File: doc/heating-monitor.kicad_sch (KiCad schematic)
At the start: 7 parts, among them U1 WeMos_D1_mini, U2 DS18B20, U3 DS18B20, U4 DS18B20, U5 DS18B20

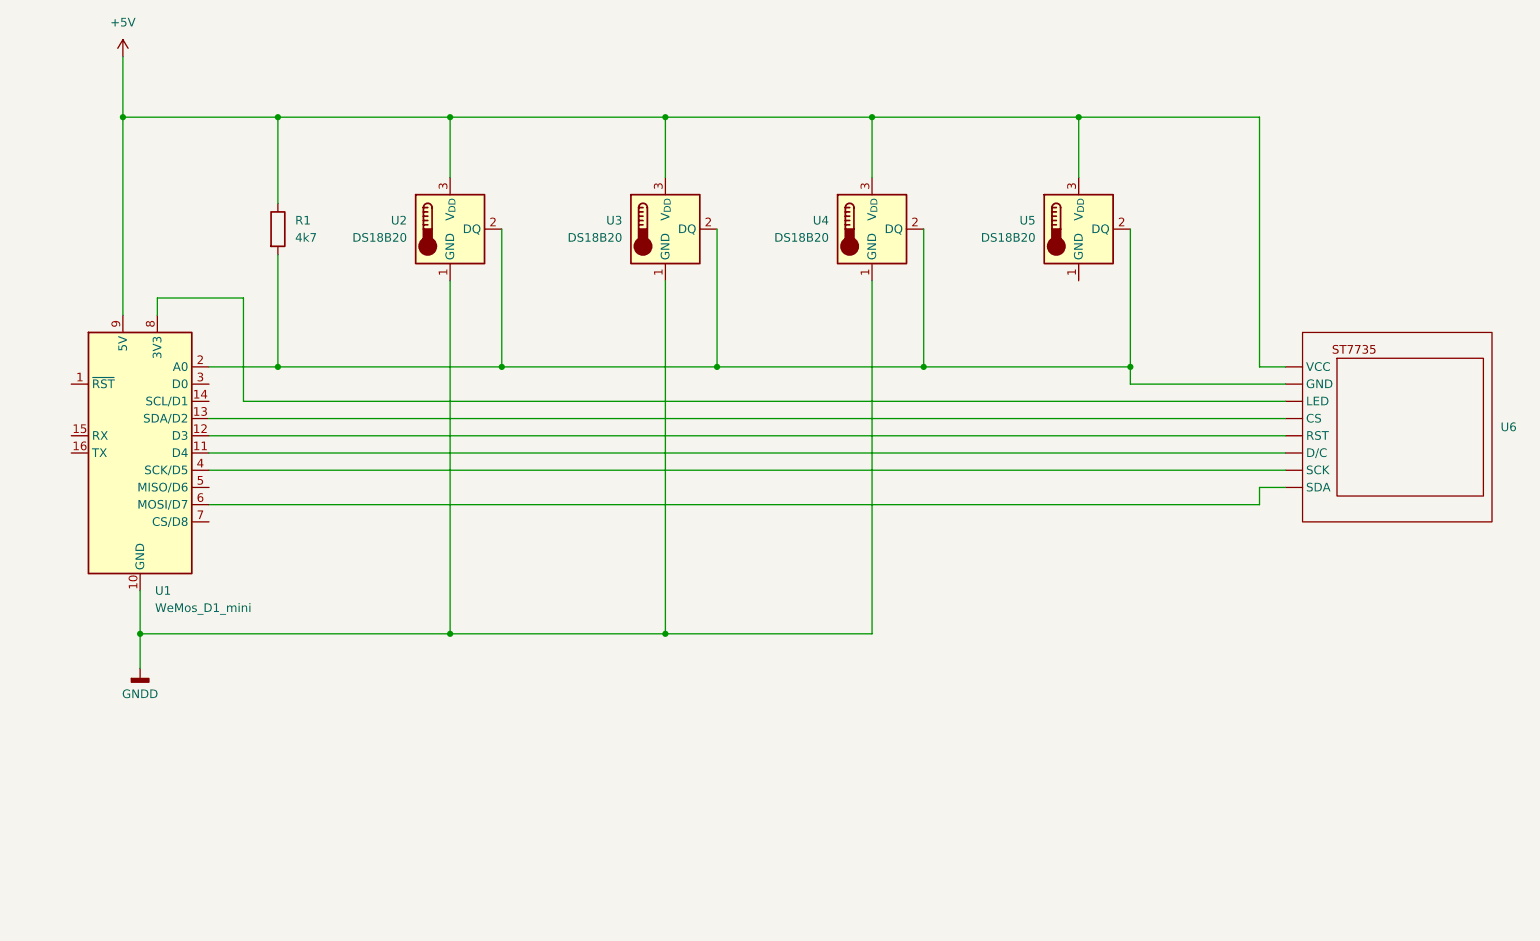
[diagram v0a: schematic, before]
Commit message: Updated schematic
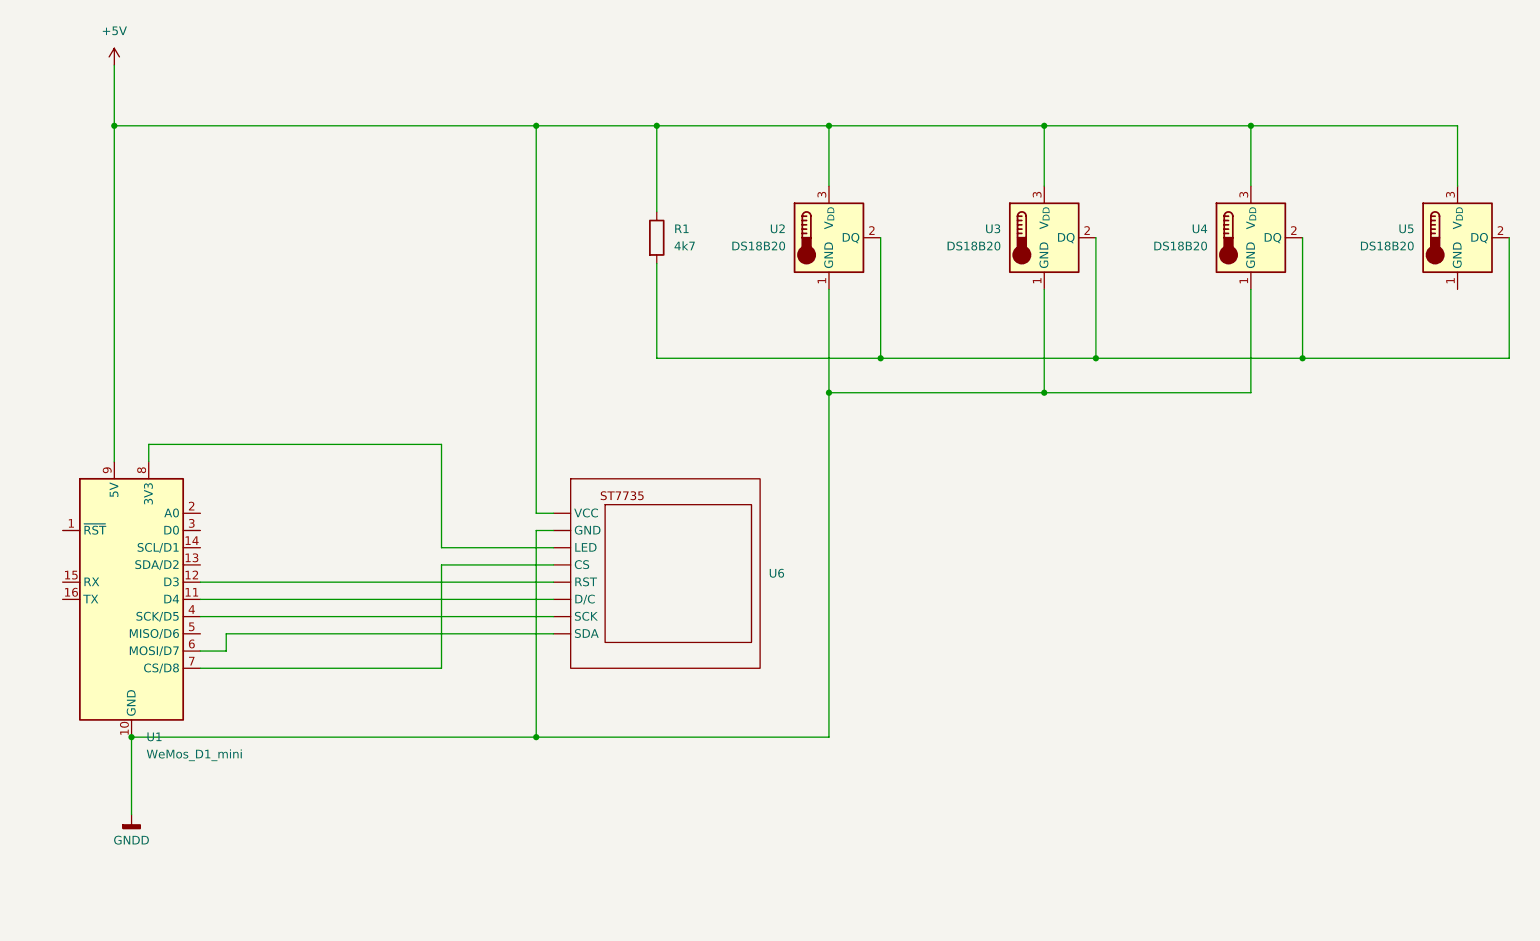
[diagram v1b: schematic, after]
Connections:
- net GNDD: now also U6. (VCC)
- net at R1.2, U2.2 (DQ), U3.2 (DQ)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: no longer U1.2 (A0), U6. (VCC)
- net at U1.13 (SDA/D2): no longer U6. (VCC)
- net at U1.7 (CS/D8): now also U6. (VCC)
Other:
- moved on the sheet: R1, U1, U2, U3, U4, U5, U6

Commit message: Update schematics
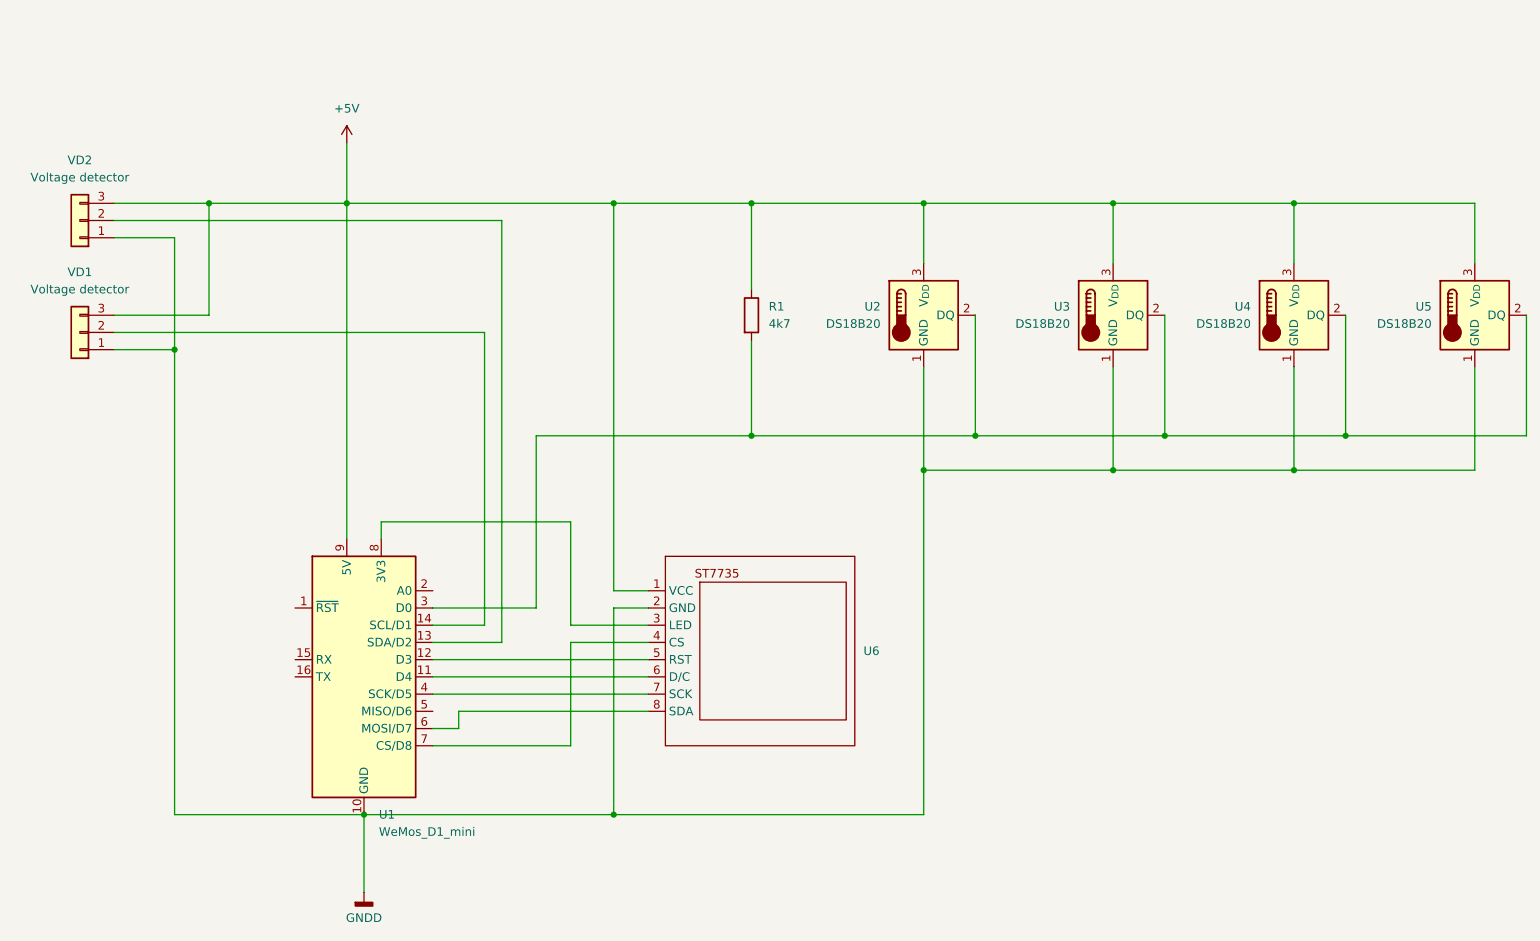
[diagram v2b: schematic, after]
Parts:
- added VD1, VD2: Voltage detector, Connector_PinHeader_2.54mm:PinHeader_1x03_P2.54mm_Vertical, symbol Connector_Generic:Conn_01x03
- R1: footprint (none) -> Resistor_THT:R_Axial_DIN0207_L6.3mm_D2.5mm_P10.16mm_Horizontal
- U6: footprint (none) -> Connector_PinHeader_2.54mm:PinHeader_1x08_P2.54mm_Vertical
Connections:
- net +5V: now also U6.1 (VCC), VD1.3 (Pin_3), VD2.3 (Pin_3); no longer U6. (VCC)
- net GNDD: now also U5.1 (GND), U6.2 (GND), VD1.1 (Pin_1), VD2.1 (Pin_1); no longer U6. (VCC)
- net at R1.2, U2.2 (DQ), U3.2 (DQ)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: now also U1.3 (D0)
- net at U1.11 (D4): now also U6.6 (D/C); no longer U6. (VCC)
- net at U1.12 (D3): now also U6.5 (RST); no longer U6. (VCC)
- net at U1.13 (SDA/D2): now also VD2.2 (Pin_2)
- net at U1.14 (SCL/D1): now also VD1.2 (Pin_2)
- net at U1.4 (SCK/D5): now also U6.7 (SCK); no longer U6. (VCC)
- net at U1.6 (MOSI/D7): now also U6.8 (SDA); no longer U6. (VCC)
- net at U1.7 (CS/D8): now also U6.4 (CS); no longer U6. (VCC)
- net at U1.8 (3V3): now also U6.3 (LED); no longer U6. (VCC)
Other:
- company: (none) -> Konajka
- title: (none) -> Heating monitor
- moved on the sheet: R1, U1, U2, U3, U4, U5
